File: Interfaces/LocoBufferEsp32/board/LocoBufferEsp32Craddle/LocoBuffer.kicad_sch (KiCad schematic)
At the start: 6 parts, among them J1 Conn_01x04, U5 ESP32-DevKitC

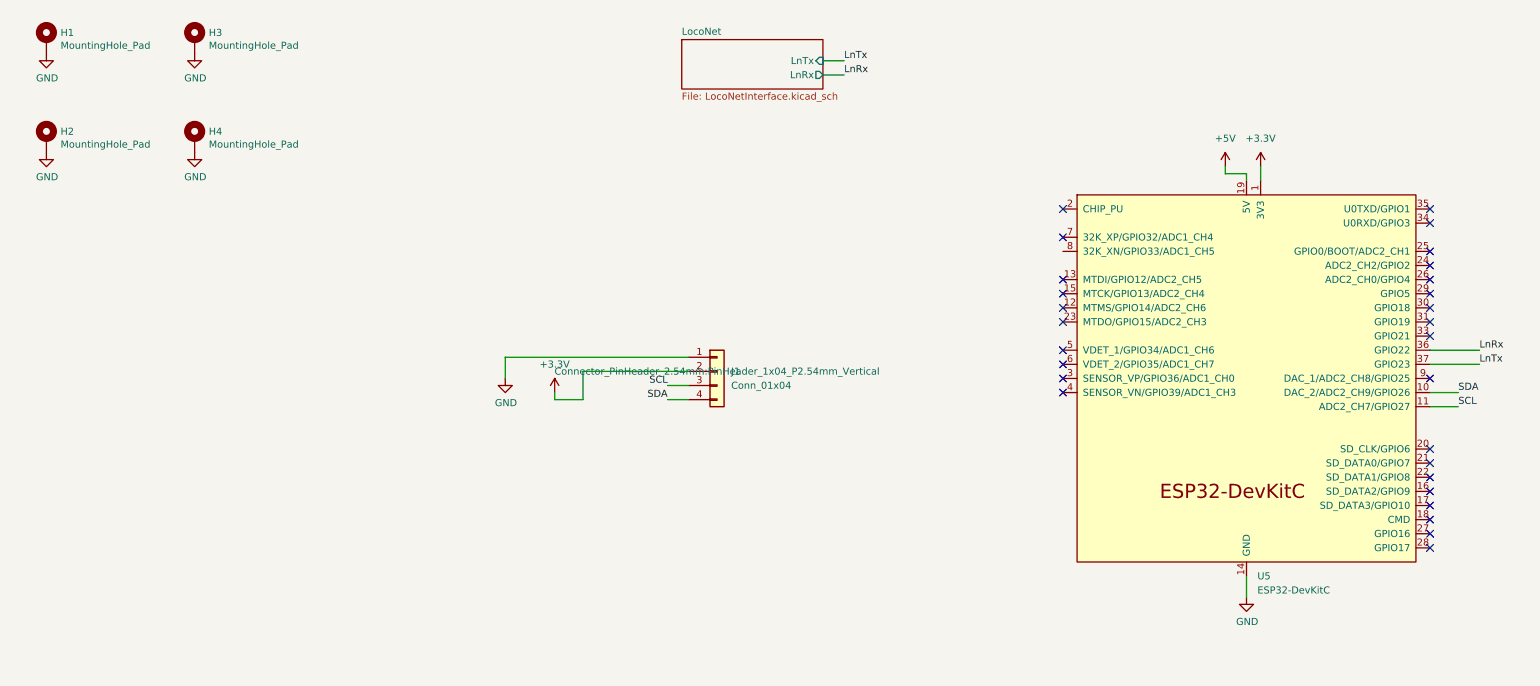
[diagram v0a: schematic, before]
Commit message: LocoCradle
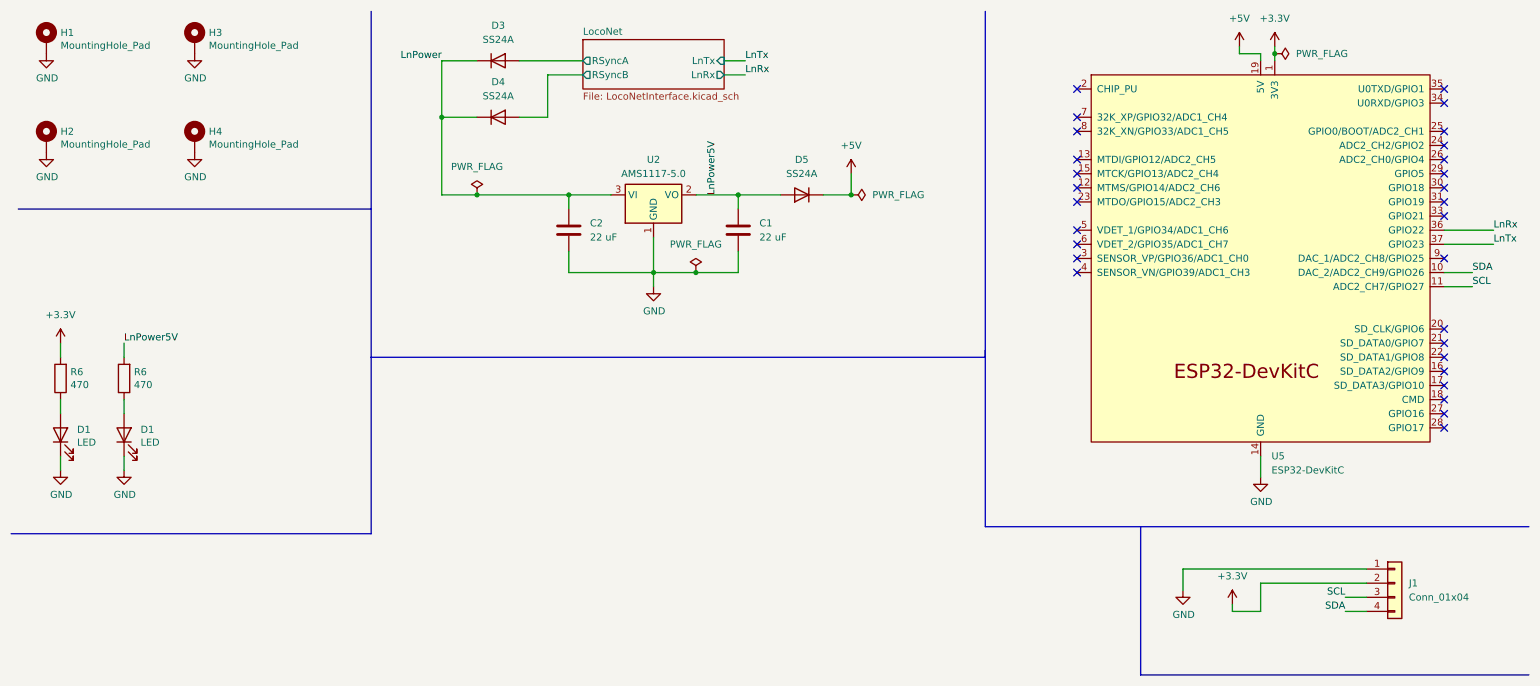
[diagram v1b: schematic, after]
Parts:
- added C1, C2: 22 uF, Capacitor_SMD:C_1206_3216Metric, symbol Device:C
- added D1 (x2): LED, LED_SMD:LED_0805_2012Metric, symbol Device:LED
- added D3, D4, D5: SS24A, Diode_SMD:D_SMA, symbol Device:D
- added R6 (x2): 470, Resistor_SMD:R_0805_2012Metric, symbol Device:R
- added U2: AMS1117-5.0, Package_TO_SOT_SMD:SOT-223-3_TabPin2, symbol Regulator_Linear:AMS1117-5.0
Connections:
- net +3.3V: now also R6.2
- net +5V: now also D5.1 (K)
- net GND: now also C1.2, C2.2, D1.1 (K), D1.1 (K), U2.1 (GND)
- new net: D1.2 (A), R6.1 (x2)
- new net LnPower: C2.1, D3.1 (K), D4.1 (K), U2.3 (VI)
- new net LnPower5V: C1.1, D5.2 (A), R6.2, U2.2 (VO)
- new net LocoNet/RSyncA: D3.2 (A)
- new net LocoNet/RSyncB: D4.2 (A)
- no-connect marks 28 -> 29
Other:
- sheet LocoNet ports: added RSyncA, RSyncB; removed none
- moved on the sheet: J1, U5
